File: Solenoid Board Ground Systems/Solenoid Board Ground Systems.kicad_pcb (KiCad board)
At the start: 2 copper layers, 58.4 x 25.4 mm, 31 parts, among them J1 OUT CHAN 1, J2 CHAN IN, J3 OUT CHAN 2

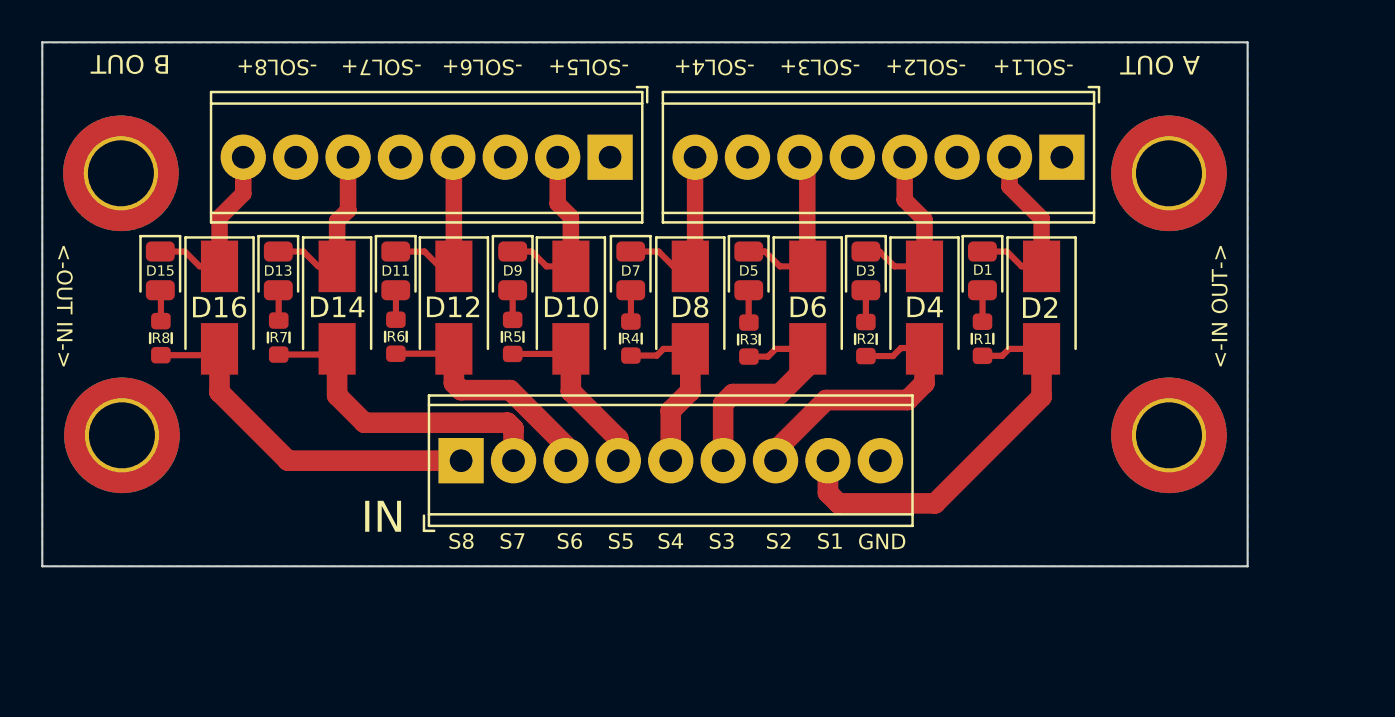
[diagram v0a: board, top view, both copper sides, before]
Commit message: Ground System Work
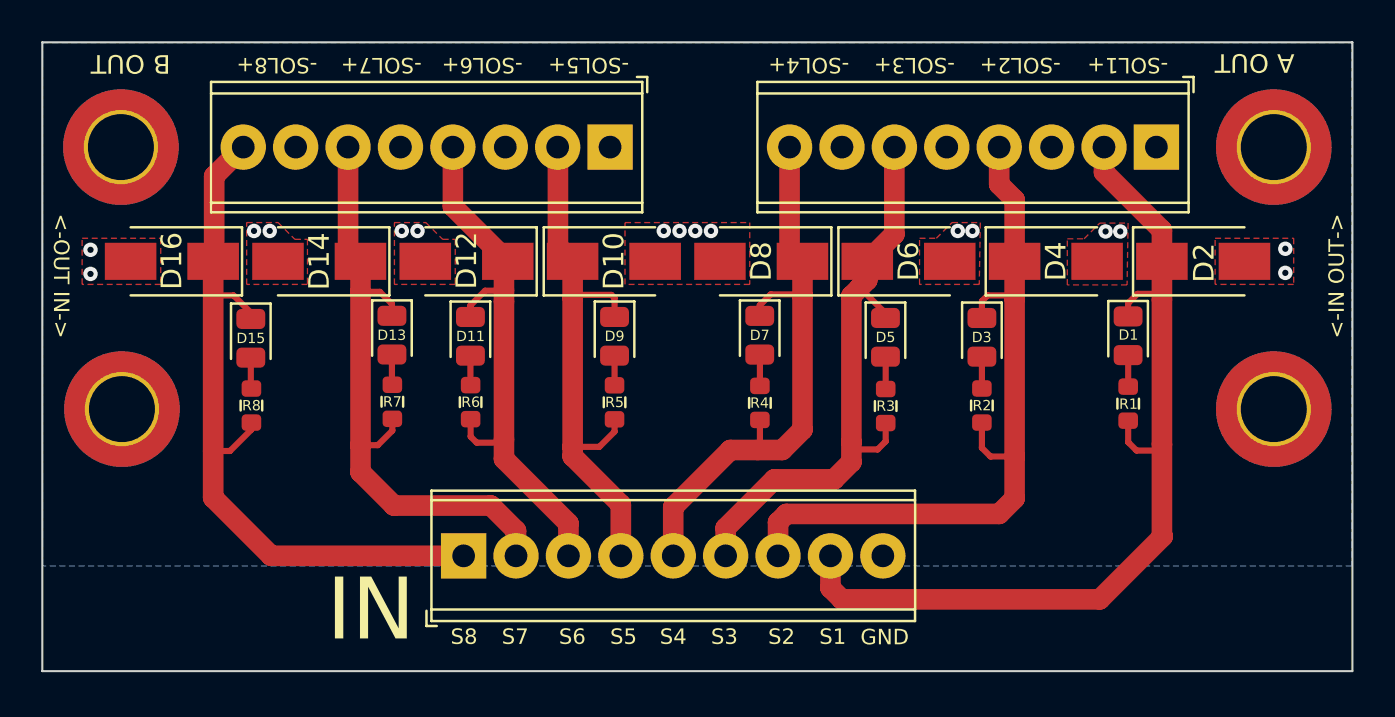
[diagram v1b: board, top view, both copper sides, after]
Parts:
- J1: value OUT CHAN 1 -> OUT CHAN A
- J2: value CHAN IN -> POWER IN
- J3: value OUT CHAN 2 -> OUT CHAN B
- moved D2 8.15 mm to (81.7, 36.0), turned to 0 degrees
- moved D1 7.73 mm to (78.0, 39.6)
- moved R1 7.73 mm to (78.0, 42.9)
- moved D5 7.37 mm to (66.3, 39.7)
- moved R3 7.37 mm to (66.3, 43.0)
- moved D7 6.99 mm to (60.2, 39.6)
- moved R4 6.99 mm to (60.2, 42.9)
- moved D4 6.75 mm to (74.5, 36.0), turned to 0 degrees
- moved D3 6.48 mm to (70.9, 39.7)
- moved R2 6.48 mm to (70.9, 43.0)
- moved D13 6.33 mm to (42.3, 39.6)
- moved R7 6.33 mm to (42.4, 42.8)
- moved D9 5.87 mm to (53.1, 39.6)
- moved R5 5.87 mm to (53.1, 42.8)
- moved D15 5.47 mm to (35.5, 39.7)
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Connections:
- D1 pad 1: Net-(D1-Pad1) -> POW IN A
- D10 pad 1: Net-(D10-Pad1) -> POW IN E
- D10 pad 2: Net-(D10-Pad2) -> GND
- D11 pad 1: Net-(D11-Pad1) -> POW IN F
- D12 pad 1: Net-(D11-Pad1) -> POW IN F
- D12 pad 2: Net-(D12-Pad2) -> GND
- D13 pad 1: Net-(D13-Pad1) -> POW IN G
- D14 pad 1: Net-(D13-Pad1) -> POW IN G
- D14 pad 2: Net-(D14-Pad2) -> GND
- D15 pad 1: Net-(D15-Pad1) -> POW IN H
- D16 pad 1: Net-(D15-Pad1) -> POW IN H
- D16 pad 2: Net-(D16-Pad2) -> GND
- D2 pad 1: Net-(D1-Pad1) -> POW IN A
- D2 pad 2: Net-(D2-Pad2) -> GND
- D3 pad 1: Net-(D3-Pad1) -> POW IN B
- D4 pad 1: Net-(D3-Pad1) -> POW IN B
- D4 pad 2: Net-(D4-Pad2) -> GND
- D5 pad 1: Net-(D5-Pad1) -> POW IN C
- D6 pad 1: Net-(D5-Pad1) -> POW IN C
- D6 pad 2: Net-(D6-Pad2) -> GND
- D7 pad 1: Net-(D7-Pad1) -> POW IN D
- D8 pad 1: Net-(D7-Pad1) -> POW IN D
- D8 pad 2: Net-(D8-Pad2) -> GND
- D9 pad 1: Net-(D10-Pad1) -> POW IN E
- J1 pad 2: Net-(D1-Pad1) -> POW IN A
- J1 pad 4: Net-(D3-Pad1) -> POW IN B
- J1 pad 6: Net-(D5-Pad1) -> POW IN C
- J1 pad 8: Net-(D7-Pad1) -> POW IN D
- J2 pad 1: Net-(D16-Pad2) -> POW IN H
- J2 pad 2: Net-(D14-Pad2) -> POW IN G
- J2 pad 3: Net-(D12-Pad2) -> POW IN F
- J2 pad 4: Net-(D10-Pad2) -> POW IN E
- J2 pad 5: Net-(D8-Pad2) -> POW IN D
- J2 pad 6: Net-(D6-Pad2) -> POW IN C
- J2 pad 7: Net-(D4-Pad2) -> POW IN B
- J2 pad 8: Net-(D2-Pad2) -> POW IN A
- J3 pad 2: Net-(D10-Pad1) -> POW IN E
- J3 pad 4: Net-(D11-Pad1) -> POW IN F
- J3 pad 6: Net-(D13-Pad1) -> POW IN G
- J3 pad 8: Net-(D15-Pad1) -> POW IN H
- R1 pad 2: Net-(D2-Pad2) -> POW IN A
- R2 pad 2: Net-(D4-Pad2) -> POW IN B
- R3 pad 2: Net-(D6-Pad2) -> POW IN C
- R4 pad 2: Net-(D8-Pad2) -> POW IN D
- R5 pad 2: Net-(D10-Pad2) -> POW IN E
- R6 pad 2: Net-(D12-Pad2) -> POW IN F
- R7 pad 2: Net-(D14-Pad2) -> POW IN G
- R8 pad 2: Net-(D16-Pad2) -> POW IN H
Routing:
- net POW IN A: track 0.00 -> 44.8 mm
- net POW IN B: track 0.00 -> 36.5 mm
- net POW IN H: track 0.00 -> 36.0 mm
- net POW IN G: track 0.00 -> 30.7 mm
- net POW IN C: track 0.00 -> 29.7 mm
- net POW IN D: track 0.00 -> 28.5 mm
- net POW IN F: track 0.00 -> 27.4 mm
- net POW IN E: track 0.00 -> 27.1 mm
- net Net-(D2-Pad2): track 19.6 -> 0.00 mm
- net Net-(D16-Pad2): track 18.2 -> 0.00 mm
- net Net-(D14-Pad2): track 16.0 -> 0.00 mm
- net Net-(D4-Pad2): track 13.7 -> 0.00 mm
- net Net-(D12-Pad2): track 12.0 -> 0.00 mm
- net Net-(D6-Pad2): track 11.5 -> 0.00 mm
- net Net-(D10-Pad2): track 9.29 -> 0.00 mm
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- added copper zone on F.Cu, net GND
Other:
- board size 58.4 x 25.4 mm -> 63.5 x 30.5 mm
